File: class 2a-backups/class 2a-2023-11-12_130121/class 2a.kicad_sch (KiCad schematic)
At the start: 32 parts, among them J1 USB_C_Receptacle, J2 Conn_01x02_Pin, J3 Conn_ARM_JTAG_SWD_10, SW1 SW_SPST, U1 STM32G030F6P6, U2 LR4054, U3 TPS613222ADBV, U4 AMS1117-3.3

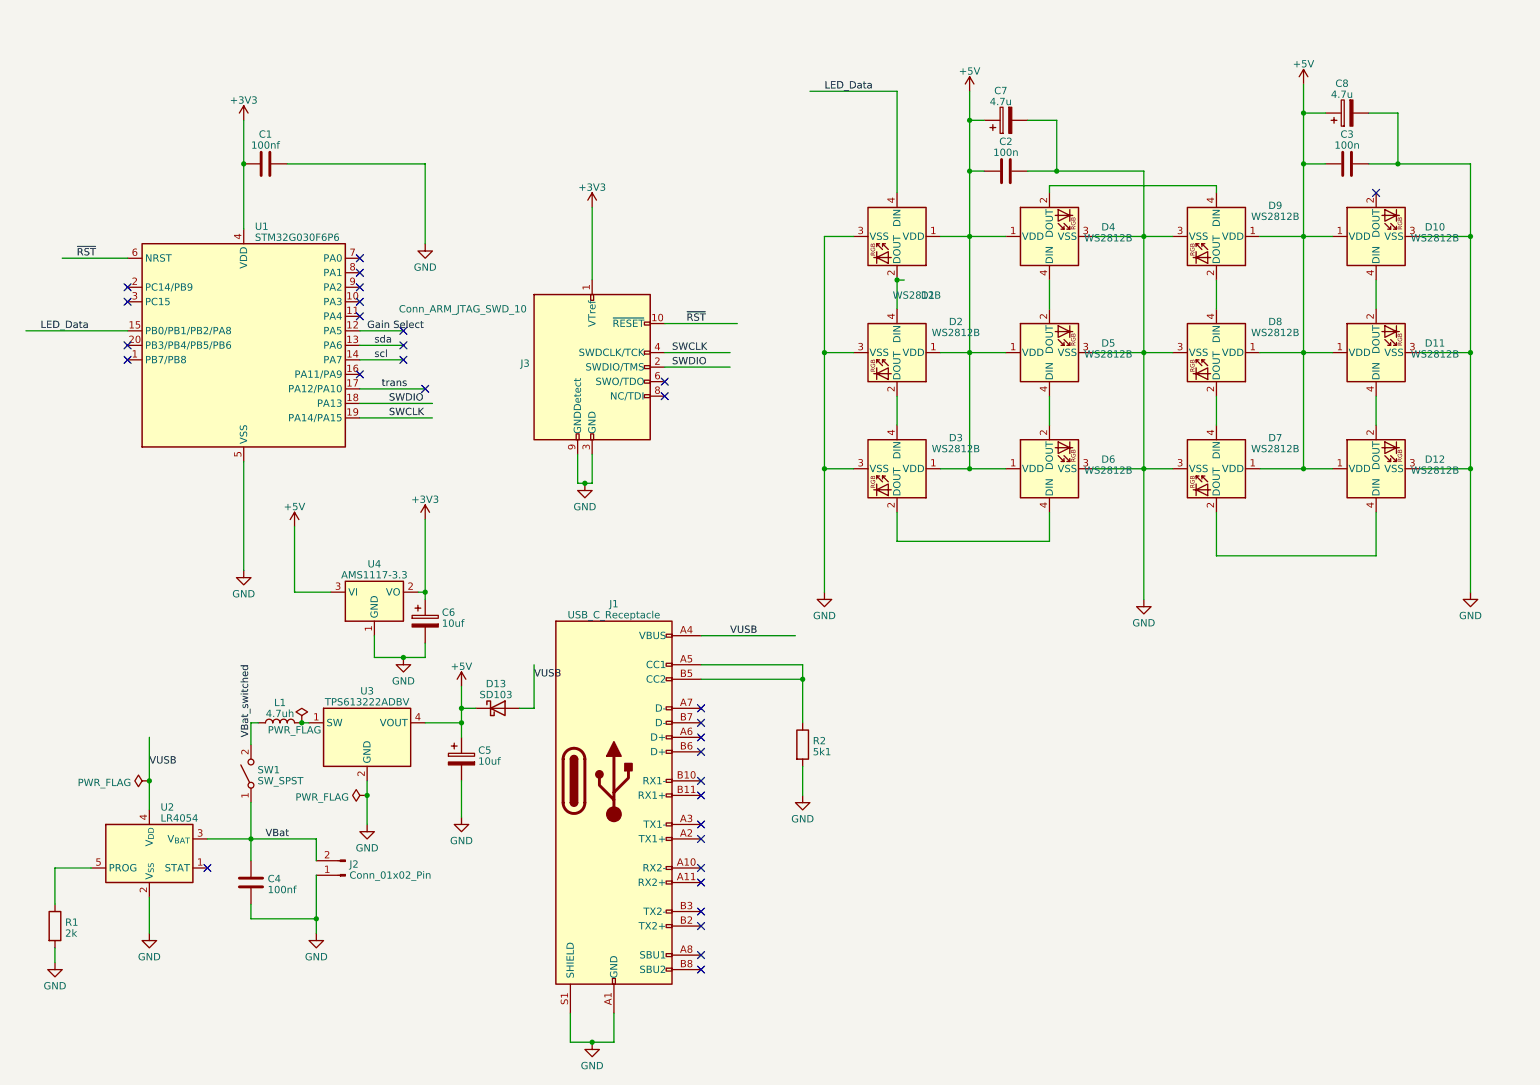
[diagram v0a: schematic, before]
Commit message: heart
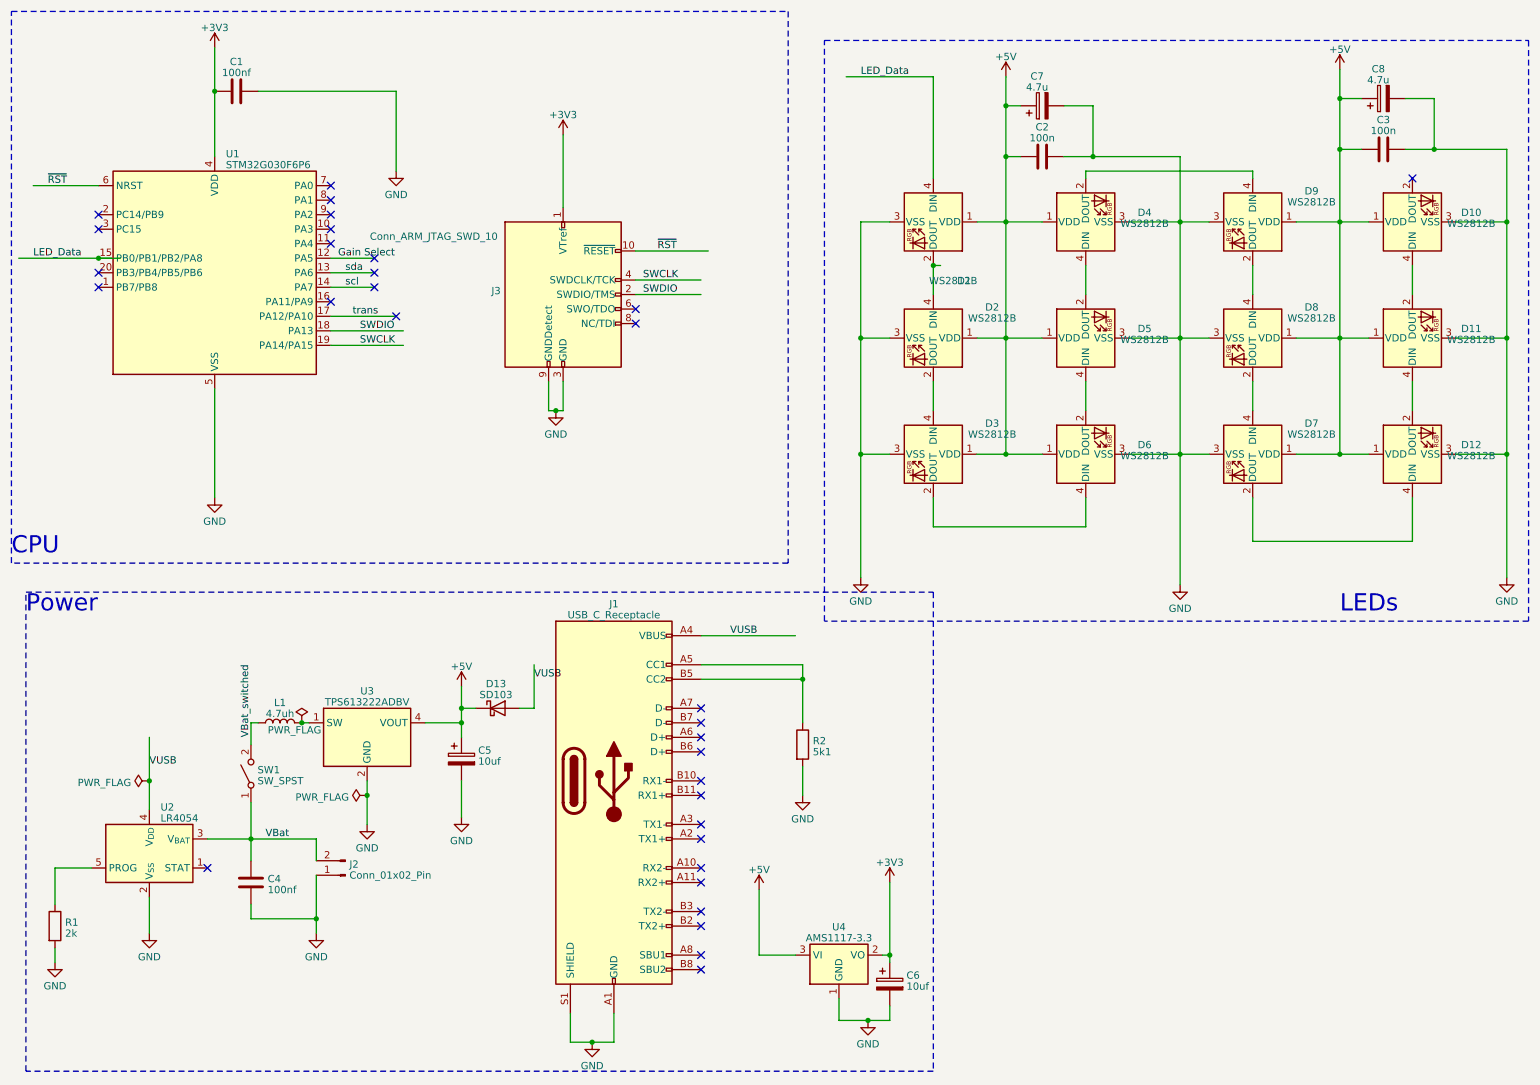
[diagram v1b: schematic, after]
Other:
- note added: "CPU"
- note added: "LEDs"
- note added: "Power"
- moved on the sheet: C1, C2, C3, C6, C7, C8, D1, D10, D11, D12, D2, D3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
